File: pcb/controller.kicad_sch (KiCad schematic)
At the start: 66 parts, among them J16 uC_NRST, J17 3V3_uC, J18 SWO, J3 CAN, J4 DEBUG, J5 UART, U2 SN65HVD234, U3 STM32F103RETx, Y1 8MHz

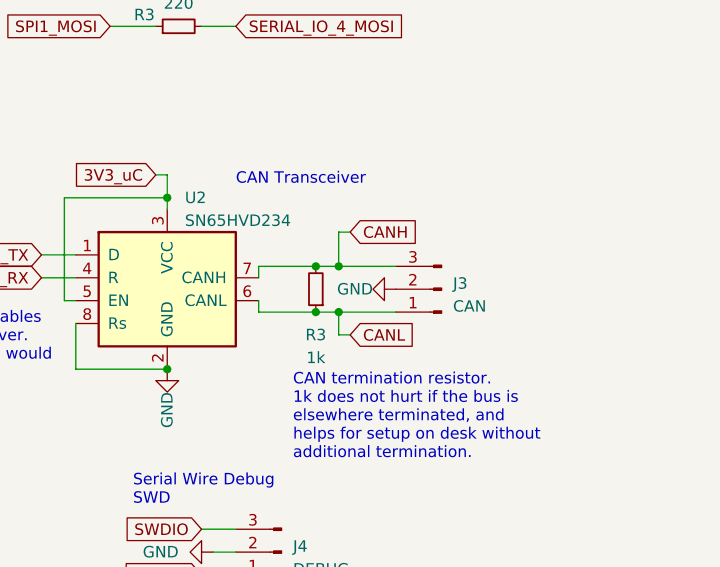
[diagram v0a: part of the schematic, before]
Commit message: added TE DEUTSCH connector and housing
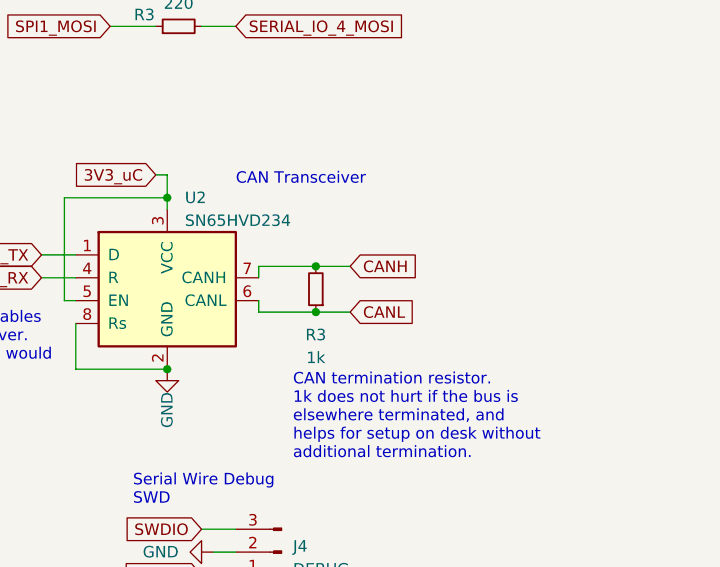
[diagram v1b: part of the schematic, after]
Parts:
- removed J3: CAN, Connector_PinHeader_2.54mm:PinHeader_1x03_P2.54mm_Vertical, symbol Connector:Conn_01x03_Pin
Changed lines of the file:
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@@
   (junction (at 161.29 57.15) (diameter 0) (color 0 0 0 0)
   )
-  (junction (at 251.46 86.36) (diameter 0) (color 0 0 0 0)
-  )
-  (junction (at 251.46 91.44) (diameter 0) (color 0 0 0 0)
-  )
   (junction (at 148.59 52.07) (diameter 0) (color 0 0 0 0)
   )
@@
     (stroke (width 0) (type default))
   )
-  (wire (pts (xy 251.46 91.44) (xy 257.81 91.44))
-    (stroke (width 0) (type default))
-  )
   (wire (pts (xy 55.88 96.52) (xy 59.69 96.52))
     (stroke (width 0) (type default))
@@
     (stroke (width 0) (type default))
   )
-  (wire (pts (xy 251.46 86.36) (xy 257.81 86.36))
-    (stroke (width 0) (type default))
-  )
   (wire (pts (xy 226.06 53.34) (xy 231.14 53.34))
     (stroke (width 0) (type default))
@@
     (stroke (width 0) (type default))
   )
-  (wire (pts (xy 252.73 93.98) (xy 251.46 93.98))
-    (stroke (width 0) (type default))
-  )
   (wire (pts (xy 123.19 69.85) (xy 135.89 69.85))
     (stroke (width 0) (type default))
@@
     (stroke (width 0) (type default))
   )
-  (wire (pts (xy 252.73 82.55) (xy 251.46 82.55))
+  (wire (pts (xy 248.92 86.36) (xy 252.73 86.36))
     (stroke (width 0) (type default))
   )
@@
     (stroke (width 0) (type default))
   )
-  (wire (pts (xy 251.46 82.55) (xy 251.46 86.36))
-    (stroke (width 0) (type default))
-  )
   (wire (pts (xy 171.45 72.39) (xy 176.53 72.39))
     (stroke (width 0) (type default))
@@
     (stroke (width 0) (type default))
   )
-  (wire (pts (xy 248.92 86.36) (xy 251.46 86.36))
-    (stroke (width 0) (type default))
-  )
   (wire (pts (xy 171.45 125.73) (xy 175.26 125.73))
     (stroke (width 0) (type default))
@@
     (stroke (width 0) (type default))
   )
-  (wire (pts (xy 251.46 93.98) (xy 251.46 91.44))
-    (stroke (width 0) (type default))
-  )
   (wire (pts (xy 171.45 92.71) (xy 175.26 92.71))
     (stroke (width 0) (type default))
@@
     (stroke (width 0) (type default))
   )
-  (wire (pts (xy 248.92 91.44) (xy 251.46 91.44))
+  (wire (pts (xy 248.92 91.44) (xy 252.73 91.44))
     (stroke (width 0) (type default))
   )
@@
     )
   )
-  (global_label "CANL" (shape input) (at 252.73 93.98 0) (fields_autoplaced)
+  (global_label "CANL" (shape input) (at 252.73 91.44 0) (fields_autoplaced)
     (effects (font (size 1.27 1.27)) (justify left))
-    (property "Intersheetrefs" "${INTERSHEET_REFS}" (at 260.353 93.98 0)
+    (property "Intersheetrefs" "${INTERSHEET_REFS}" (at 260.353 91.44 0)
       (effects (font (size 1.27 1.27)) (justify left) hide)
     )
   )
-  (global_label "CANH" (shape input) (at 252.73 82.55 0) (fields_autoplaced)
+  (global_label "CANH" (shape input) (at 252.73 86.36 0) (fields_autoplaced)
     (effects (font (size 1.27 1.27)) (justify left))
-    (property "Intersheetrefs" "${INTERSHEET_REFS}" (at 260.6554 82.55 0)
+    (property "Intersheetrefs" "${INTERSHEET_REFS}" (at 260.6554 86.36 0)
       (effects (font (size 1.27 1.27)) (justify left) hide)
     )
@@
     )
   )
-  (symbol (lib_id "Connector:Conn_01x03_Pin") (at 262.89 88.9 180) (unit 1)
-    (in_bom yes) (on_board yes) (dnp no) (fields_autoplaced)
-    (property "Reference" "J3" (at 264.16 88.265 0)
-      (effects (font (size 1.27 1.27)) (justify right))
-    )
-    (property "Value" "CAN" (at 264.16 90.805 0)
-      (effects (font (size 1.27 1.27)) (justify right))
-    )
-    (property "Footprint" "Connector_PinHeader_2.54mm:PinHeader_1x03_P2.54mm_Vertical" (at 262.89 88.9 0)
-      (effects (font (size 1.27 1.27)) hide)
-    )
-    (property "Datasheet" "~" (at 262.89 88.9 0)
-      (effects (font (size 1.27 1.27)) hide)
-    )
-    (pin "1")
-    (pin "2")
-    (pin "3")
-    (instances
-      (project "qca7000"
-        (path "/e63e39d7-6ac0-4ffd-8aa3-1841a4541b55/5666e7cf-6b6c-4583-8335-aa3be69ccd45"
-          (reference "J3") (unit 1)
-        )
-      )
-    )
-  )
   (symbol (lib_id "Connector:Conn_01x03_Pin") (at 256.54 154.94 180) (unit 1)
     (in_bom yes) (on_board yes) (dnp no) (fields_autoplaced)
@@
         )
       )
-    )
-  )
-  (symbol (lib_id "power:GND") (at 257.81 88.9 270) (unit 1)
-    (in_bom yes) (on_board yes) (dnp no)
-    (property "Reference" "#PWR048" (at 251.46 88.9 0)
-      (effects (font (size 1.27 1.27)) hide)
-    )
-    (property "Value" "GND" (at 255.27 88.9 90)
-      (effects (font (size 1.27 1.27)) (justify right))
-    )
-    (property "Footprint" "" (at 257.81 88.9 0)
-      (effects (font (size 1.27 1.27)) hide)
-    )
-    (property "Datasheet" "" (at 257.81 88.9 0)
-      (effects (font (size 1.27 1.27)) hide)
-    )
-    (pin "1")
-    (instances
-      (project "qca7000"
-        (path "/e63e39d7-6ac0-4ffd-8aa3-1841a4541b55"
-          (reference "#PWR048") (unit 1)
-        )
-        (path "/e63e39d7-6ac0-4ffd-8aa3-1841a4541b55/5666e7cf-6b6c-4583-8335-aa3be69ccd45"
-          (reference "#PWR049") (unit 1)
-        )
-      )
